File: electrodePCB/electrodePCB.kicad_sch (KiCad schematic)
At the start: 20 parts, among them J1 FPC 20p, J2 qwiic, U1 TMP119AIYBGR

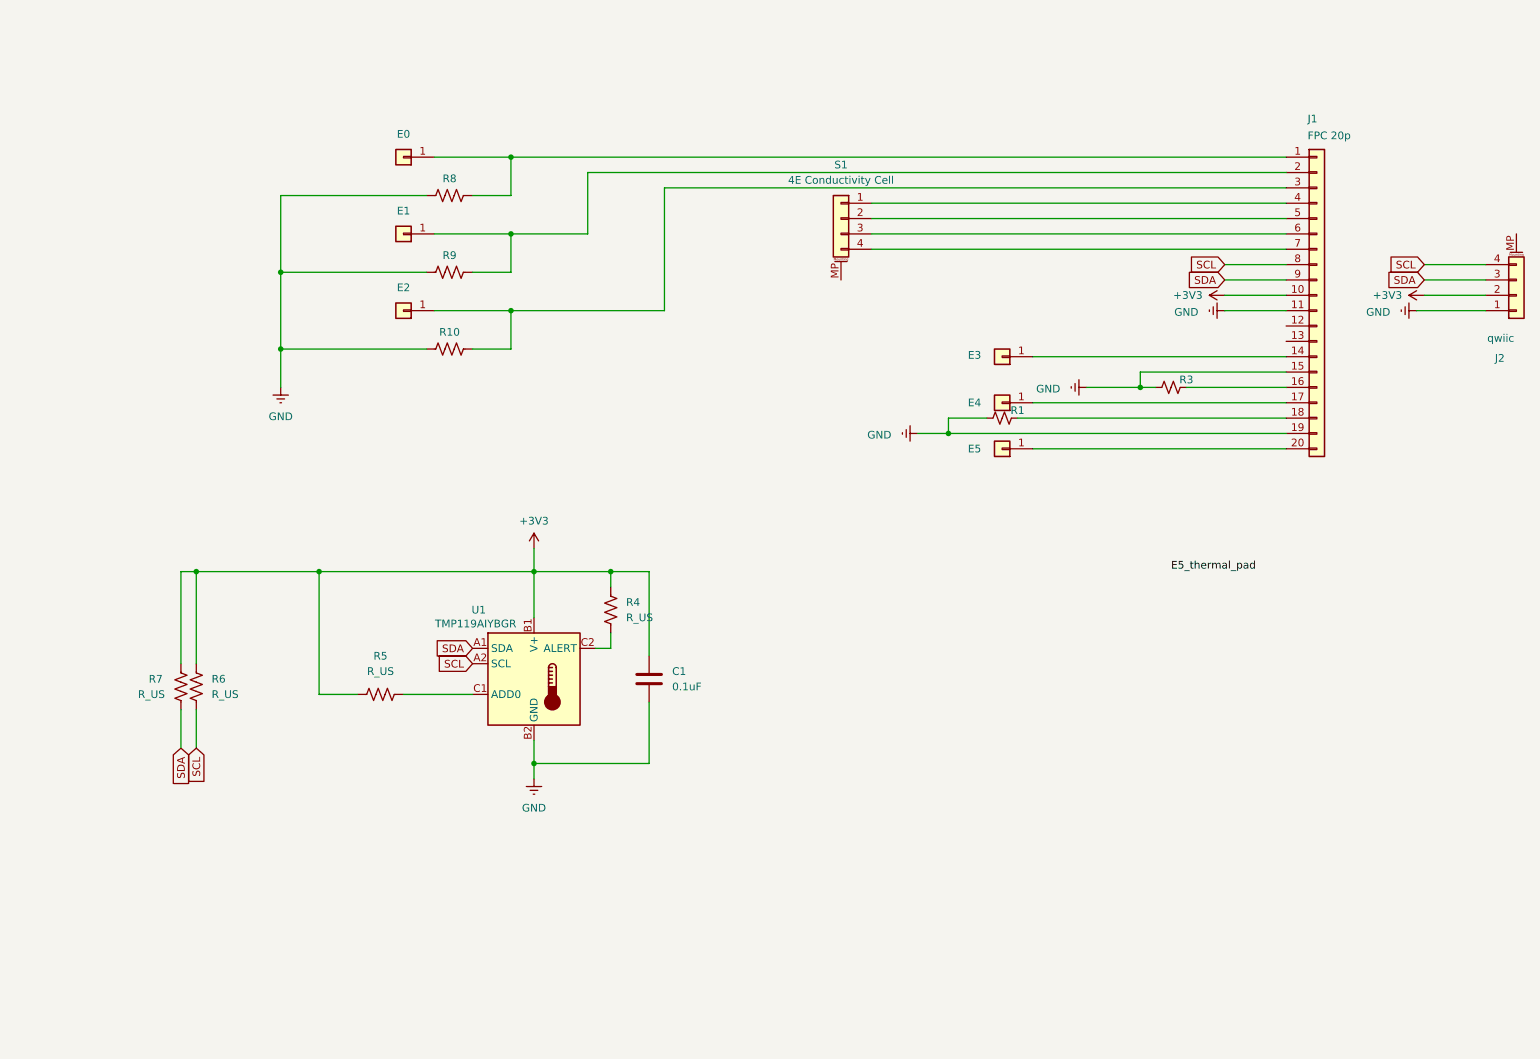
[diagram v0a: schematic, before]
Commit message: roughly finalized layout. Might tidy up the GND plane with some keep outs
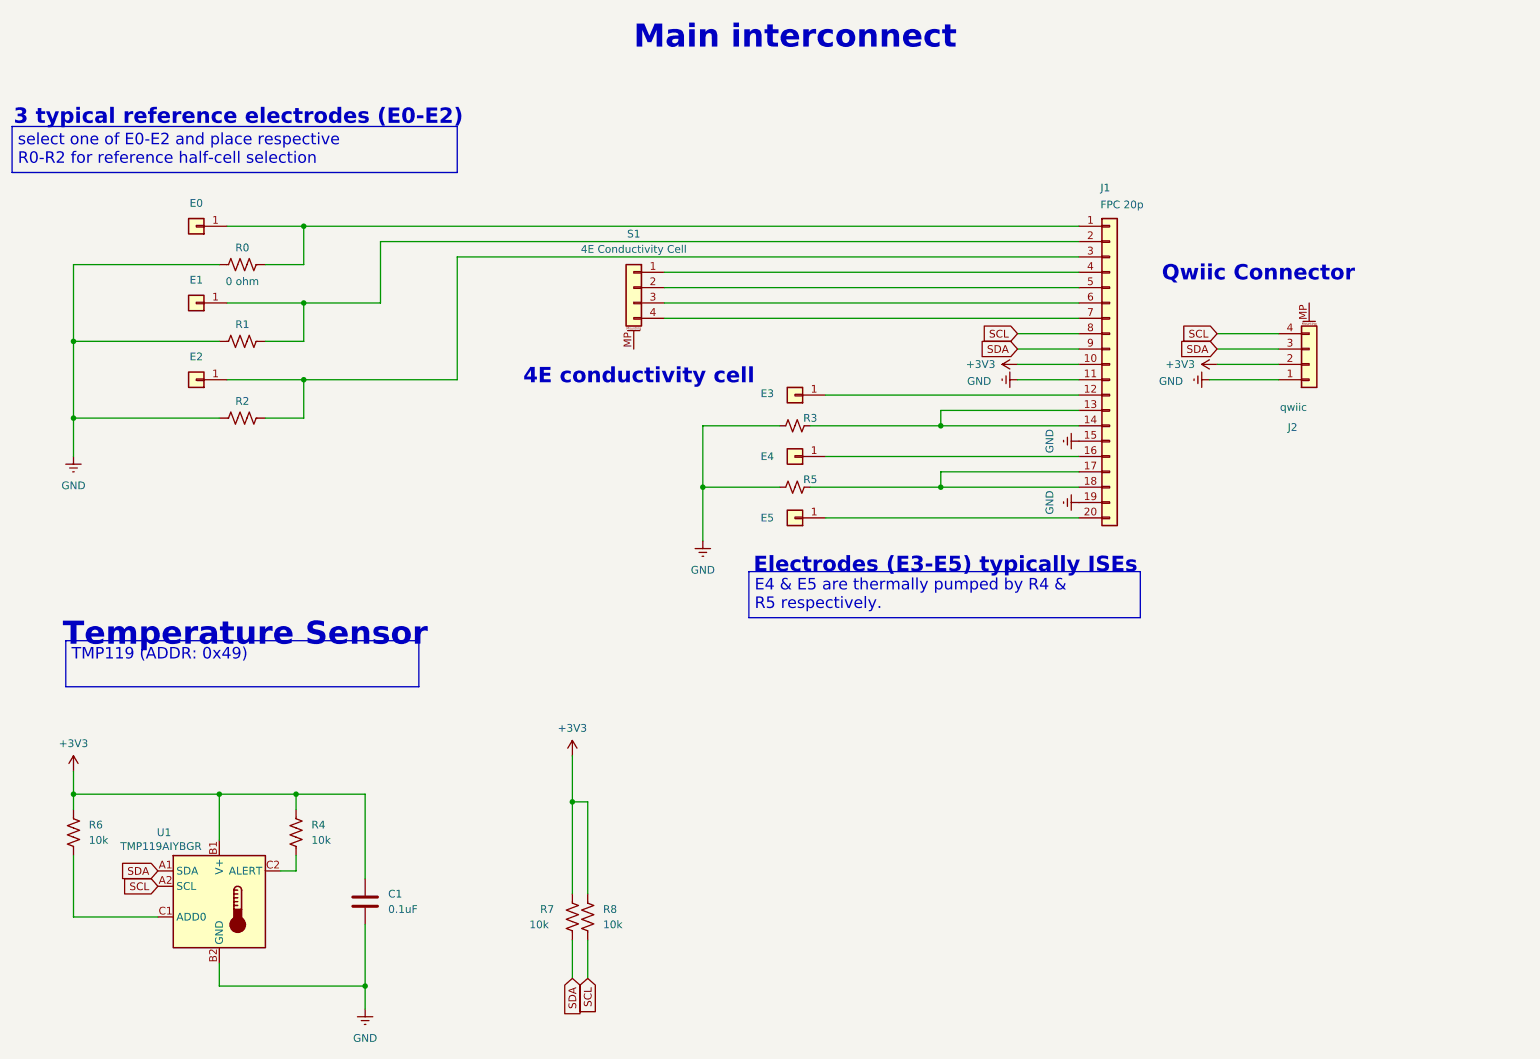
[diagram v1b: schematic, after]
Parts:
- R0: renamed from R8; value R_US -> 0 ohm
- R4, R7: value R_US -> 10k
- R6: renamed from R5; value R_US -> 10k
- R8: renamed from R6; value R_US -> 10k
- renumbered R9 to R1, R10 to R2, R1 to R5
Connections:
- net at E3.1 (Pin_1): now also J1.12 (Pin_12); no longer J1.14 (Pin_14)
- net at J1.18 (Pin_18), R5.1: now also J1.17 (Pin_17)
- net at E4.1 (Pin_1): now also J1.16 (Pin_16); no longer J1.17 (Pin_17)
- net at R3.1: now also J1.13 (Pin_13), J1.14 (Pin_14); no longer J1.16 (Pin_16)
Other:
- note added: "3 typical reference electrodes (E0-E2)"
- note added: "4E conductivity cell"
- note added: "Electrodes (E3-E5) typically ISEs"
- note added: "Main interconnect"
- note added: "Qwiic Connector"
- note added: "Temperature Sensor"
- company: (none) -> William Pardis
- title: (none) -> electrodePCB
- moved on the sheet: C1, E0, E1, E2, E3, E4, E5, J1, J2, R0, R1, R2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
